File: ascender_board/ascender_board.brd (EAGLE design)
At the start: 94 x 80 mm, 89 parts, among them Q1 8MHz, U1 STM32F722XX, U2 LM5107MA, U3 LM5107MA, U4 LM5107MA, U5 LM5107MA, U6 LM5107MA, U7 LM5107MA, X1 MINI-USB-32005-201

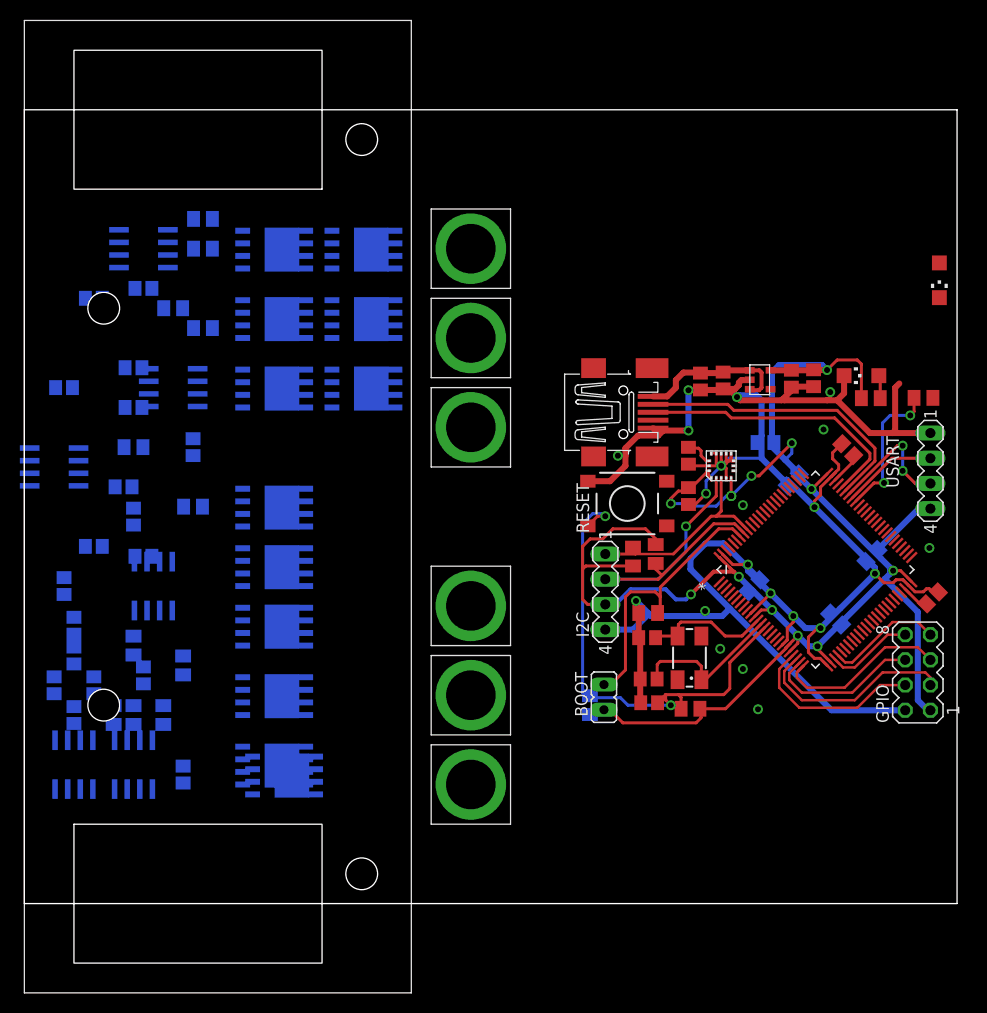
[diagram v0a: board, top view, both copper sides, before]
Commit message: board
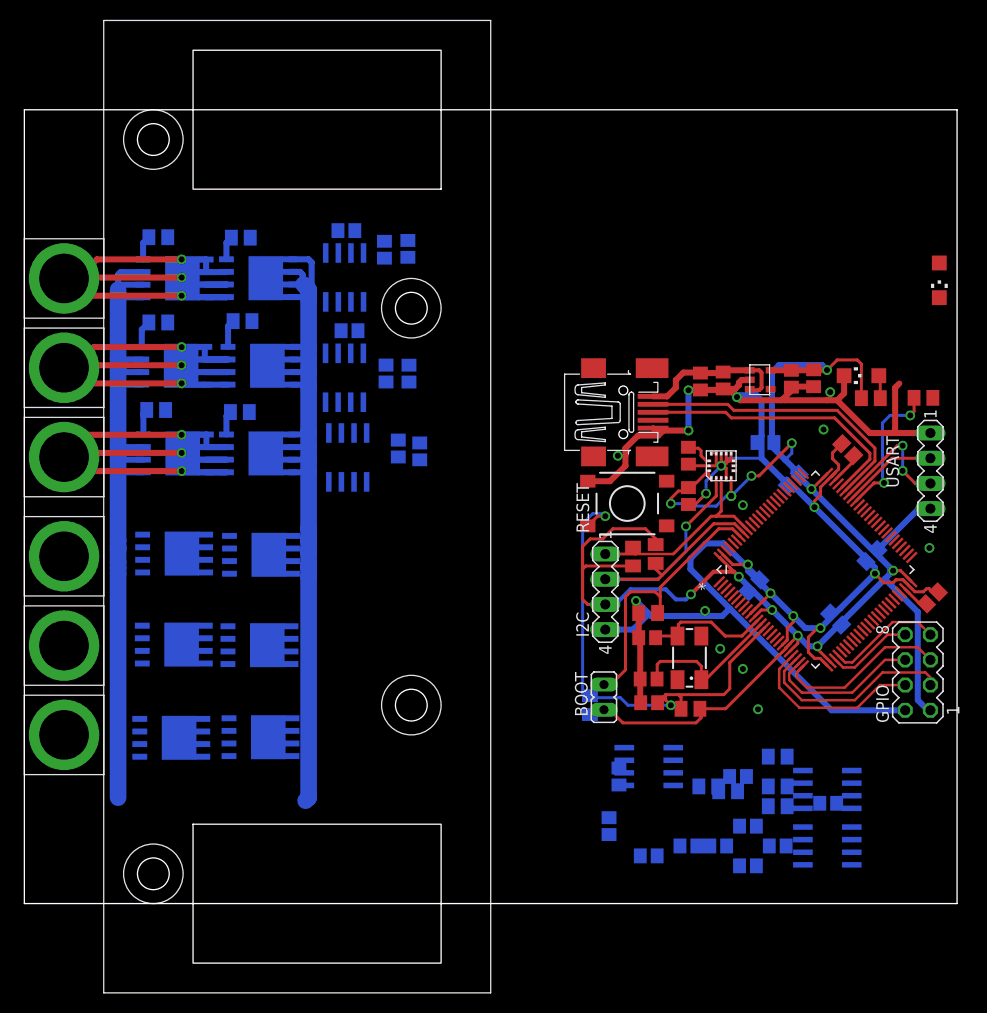
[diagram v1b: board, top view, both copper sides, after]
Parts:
- moved U5 76.4 mm to (80.9, 5.81), turned to 0 degrees
- moved C34 72.3 mm to (72.9, 3.81), turned to 0 degrees
- moved C32 72.1 mm to (75.9, 5.81), turned to 0 degrees
- moved U7 70.0 mm to (80.9, 11.5), turned to 0 degrees
- moved C26 67.7 mm to (69.9, 5.81), turned to 0 degrees
- moved R14 67.6 mm to (75.9, 9.81), turned to 0 degrees
- moved C28 67.4 mm to (72.9, 7.81), turned to 0 degrees
- moved C30 65.8 mm to (66.9, 5.81), turned to 0 degrees
- moved R13 65.3 mm to (75.9, 11.8), turned to 0 degrees
- moved C33 65.1 mm to (81.0, 10.1), turned to 0 degrees
- moved C31 64.9 mm to (62.9, 4.81), turned to 0 degrees
- moved R16 62.1 mm to (75.9, 14.8), turned to 0 degrees
- moved C27 60.8 mm to (71.9, 12.8), turned to 0 degrees
- moved R15 59.6 mm to (68.9, 11.8), turned to 0 degrees
- moved C25 59.1 mm to (58.9, 7.81), turned to 270 degrees
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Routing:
- net VCC: track 0.00 -> 81.3 mm
- net GND: track 226.9 -> 304.9 mm
- net N$25: track 0.00 -> 60.5 mm, vias 0 -> 3
- net N$19: track 0.00 -> 59.9 mm, vias 0 -> 3
- net N$16: track 0.00 -> 59.1 mm, vias 0 -> 3
- net N$17: track 0.00 -> 2.81 mm
- net N$7: track 0.00 -> 2.76 mm
- net N$20: track 0.00 -> 2.61 mm
- net N$8: track 0.00 -> 2.49 mm
- net N$23: track 0.00 -> 2.43 mm
- net N$12: track 0.00 -> 2.38 mm
